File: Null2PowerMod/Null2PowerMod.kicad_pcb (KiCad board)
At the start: 2 copper layers, 18 x 28 mm, 32 parts, among them J1 Conn_01x01, J2 USB_C_Receptacle_USB2.0, J3 Conn_01x01, J5 JST 2-PH, J6 Conn_01x01, U1 MCP73871, U2 TPS61030PWP

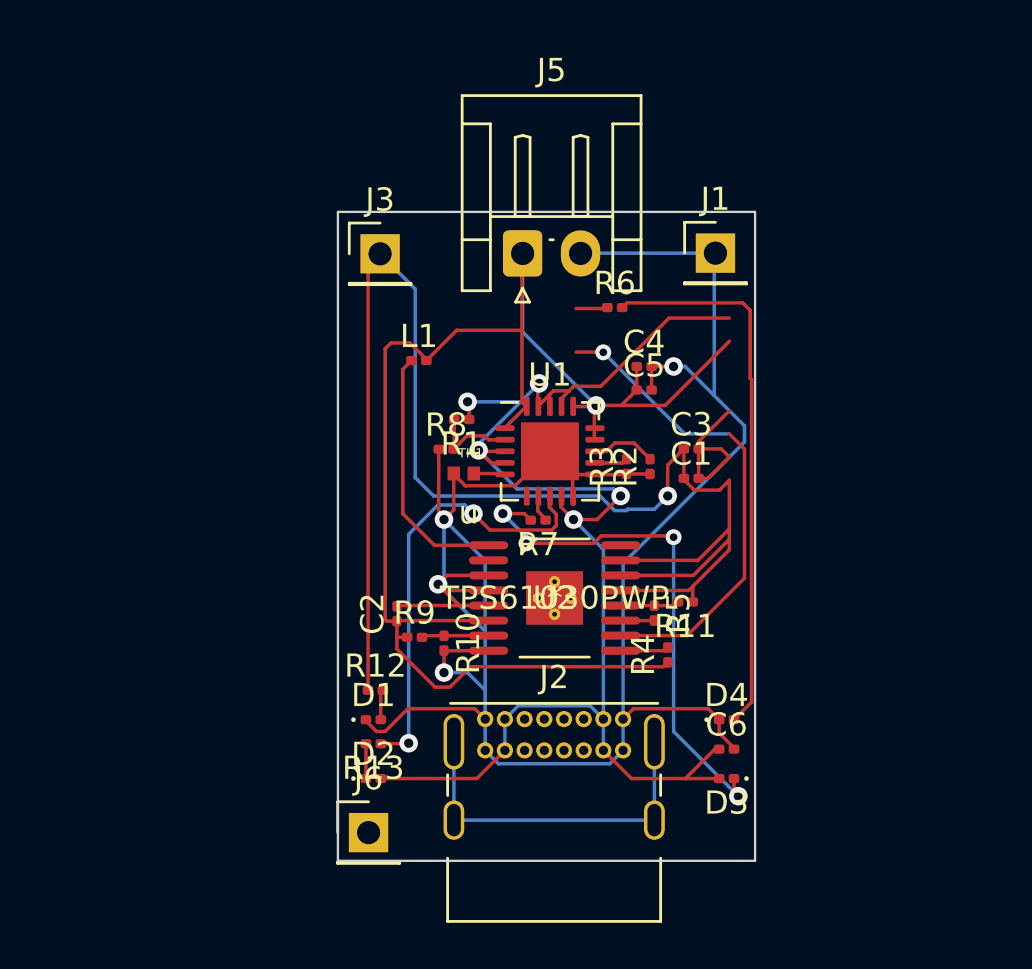
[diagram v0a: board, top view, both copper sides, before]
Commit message: wtf happened to the schematic?
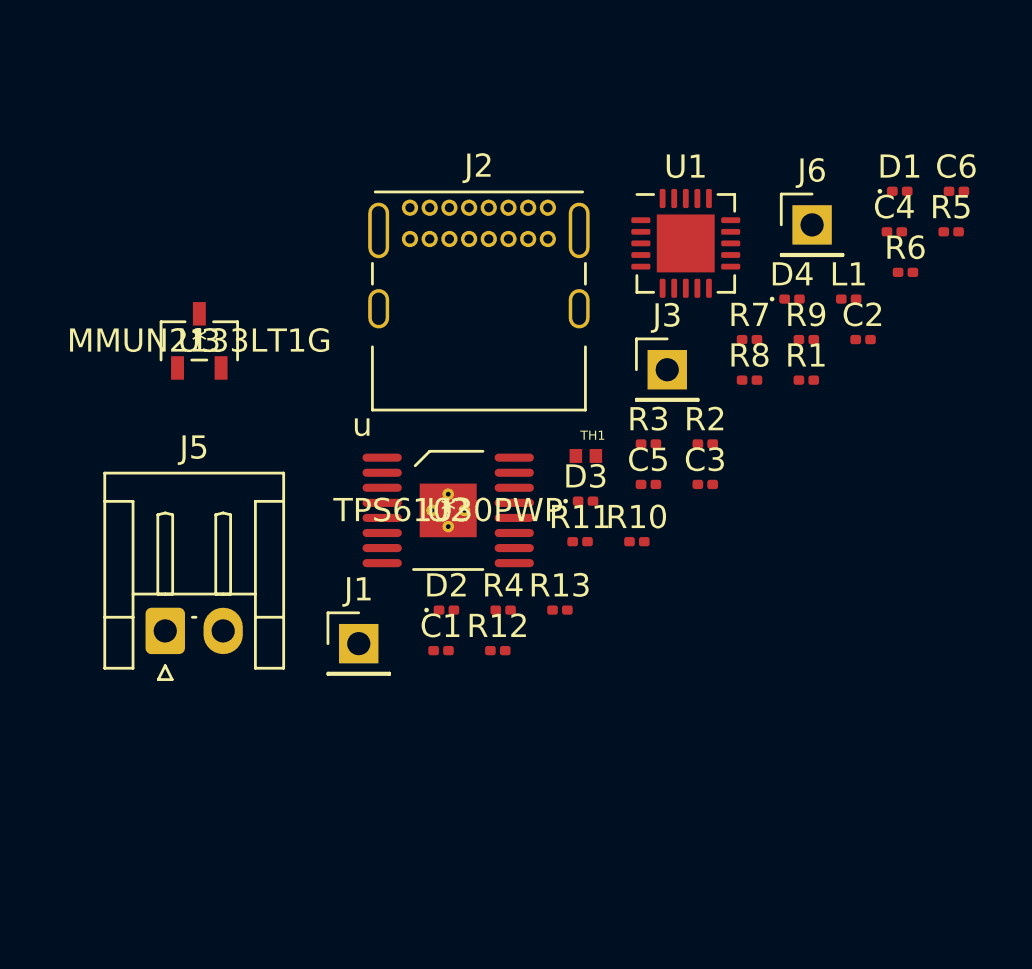
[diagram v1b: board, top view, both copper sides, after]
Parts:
- added U3: MMUN2133LT1G, MMUN2133LT1G:MMUN2133LT1G, F.Cu at (89.0, 44.6)
- moved J6 32.5 mm to (115.5, 39.6)
- moved D1 32.2 mm to (119.2, 38.2)
- moved C6 26.0 mm to (121.7, 38.2)
- moved C2 23.3 mm to (117.7, 44.6), turned to 0 degrees
- moved J1 22.8 mm to (95.9, 57.7)
- moved J5 22.4 mm to (87.5, 57.1)
- moved J2 22.3 mm to (98.1, 38.9)
- moved R9 21.2 mm to (115.2, 44.6)
- moved R5 20.8 mm to (121.5, 39.9), turned to 0 degrees
- moved L1 18.7 mm to (117.0, 42.8)
- moved D4 18.4 mm to (114.6, 42.8)
- moved R1 15.0 mm to (115.2, 46.3), turned to 0 degrees
- moved D3 13.4 mm to (105.7, 51.5), turned to 0 degrees
- moved R8 13.4 mm to (112.8, 46.3)
- moved J3 13.4 mm to (109.2, 45.9)
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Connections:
- C2 pad 1: VLIPO -> Net-(C2-Pad1)
- C3 pad 1: VLIPO -> Net-(C3-Pad1)
- C4 pad 1: VLIPO -> Net-(C3-Pad1)
- J3 pad 1: VLIPO -> VBUS
- L1 pad 2: VLIPO -> VBAT
- R7 pad 1: VLIPO -> unconnected-(R7-Pad1)
- R8 pad 1: VLIPO -> Net-(C3-Pad1)
- U1 pad 1: VLIPO -> Net-(U1-Pad1)
- U1 pad 14: VLIPO -> Net-(C2-Pad1)
- U1 pad 15: VLIPO -> Net-(C2-Pad1)
- U1 pad 16: VLIPO -> Net-(C2-Pad1)
- U1 pad 20: VLIPO -> Net-(U1-Pad1)
- U2 pad 6: VLIPO -> Net-(C3-Pad1)
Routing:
- net GND: track 135.8 -> 0.00 mm, vias 5 -> 0
- net +5V: track 128.9 -> 0.00 mm, vias 1 -> 0
- net VLIPO: track 74.0 -> 0.00 mm, vias 1 -> 0
- net Net-(D2-Pad1): track 23.7 -> 0.00 mm
- net Net-(R13-Pad1): track 19.0 -> 0.00 mm
- net (no net): track 15.4 -> 0.00 mm
- net /LB0: track 12.9 -> 0.00 mm, vias 1 -> 0
- net Net-(L1-Pad1): track 11.0 -> 0.00 mm
- net Net-(R2-Pad2): track 4.93 -> 0.00 mm
- net Net-(R8-Pad2): track 3.76 -> 0.00 mm
- net Net-(D4-Pad2): track 1.50 -> 0.00 mm
- net Net-(R3-Pad2): track 1.46 -> 0.00 mm
- net Net-(R6-Pad1): track 1.36 -> 0.00 mm, vias 2 -> 0
- net Net-(TH1-Pad2): track 1.34 -> 0.00 mm
- net Net-(D3-Pad2): track 1.31 -> 0.00 mm
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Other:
- board outline removed
